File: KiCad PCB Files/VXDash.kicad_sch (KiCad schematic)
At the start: 15 parts, among them IC1 CD74HC4050M96, IC2 SP721ABG, IC5 74HC4067BQ-Q100J, J1 MX34036UF2, J2 Conn_01x04_Socket, K1 G6L-1P-DC12, K2 G6L-1P-DC12

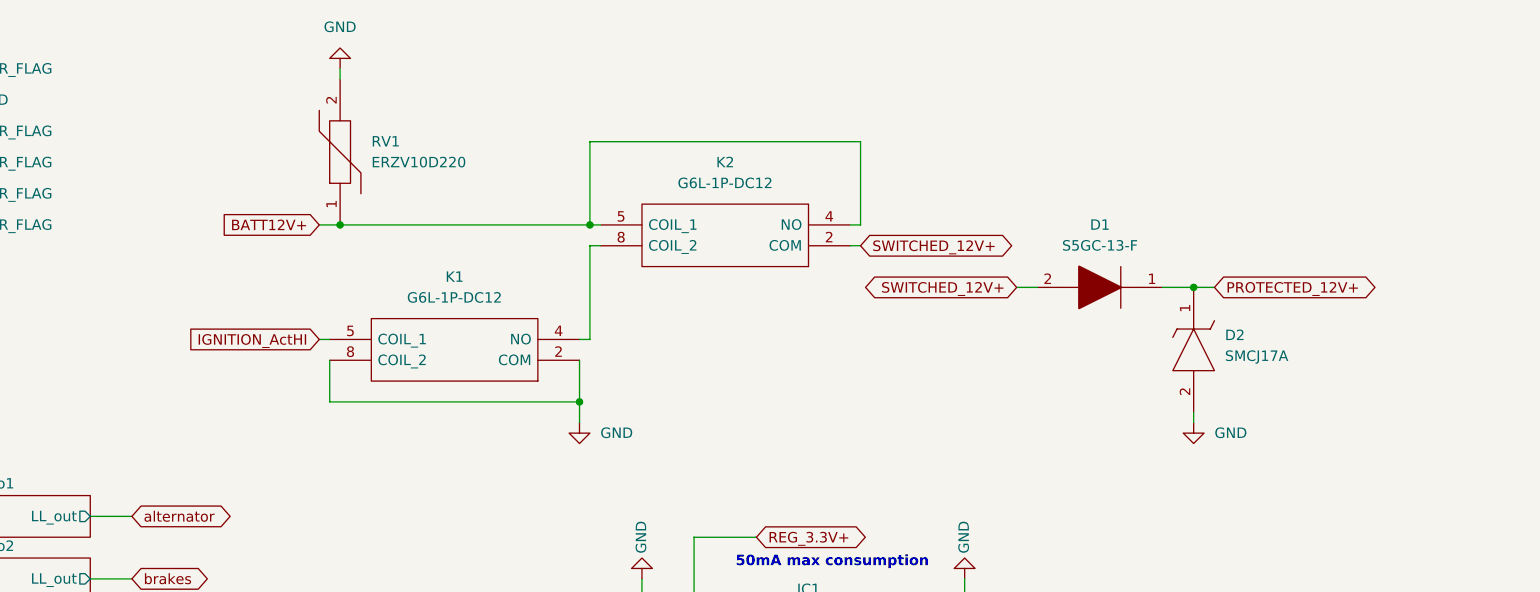
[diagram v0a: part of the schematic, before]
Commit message: Added power input sch
Added power input sheet.
Relays removed.
MOSFETs added for switching power.
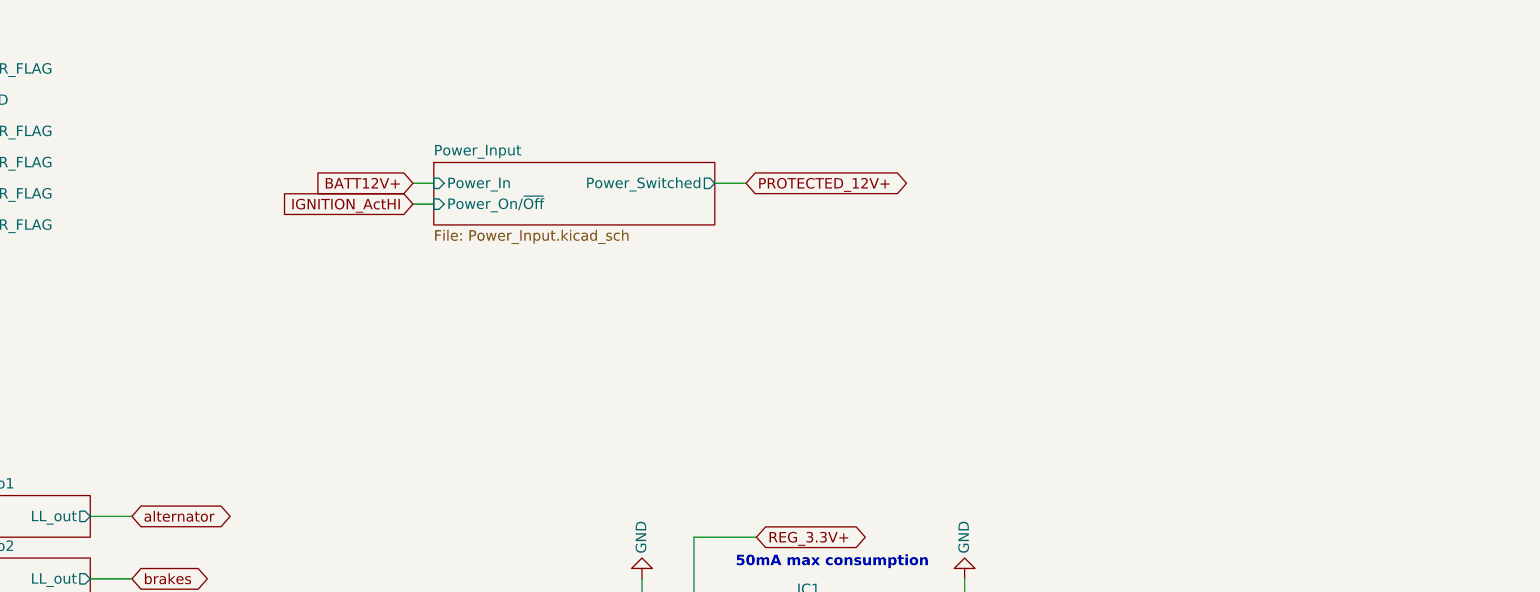
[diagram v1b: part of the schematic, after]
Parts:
- removed D1: S5GC-13-F, Diode_SMD:D_SMC, symbol SamacSys_Parts:S5GC-13-F
- removed D2: SMCJ17A, Diode_SMD:D_SMC, symbol SamacSys_Parts:SMCJ17A
- removed K1, K2: G6L-1P-DC12, SamacSys_Parts:G6L-1P_2, symbol SamacSys_Parts:G6L-1P-DC12
- removed RV1: ERZV10D220, SamacSys_Parts:ERZV10D220, symbol SamacSys_Parts:ERZV10D220
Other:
- added sheet Power_Input (Power_Input.kicad_sch)
